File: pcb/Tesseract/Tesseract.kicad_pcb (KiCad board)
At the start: 2 copper layers, 67 x 55 mm, 31 parts, among them IC1 MAX98357AETE+T, J1 NHD-1.91-176176UBC3 Conn-1, J2 USB C Power Connector, J3 Speaker Connector, J4 RPI Power Connector, J5 LED Strip Connector, J6 RPI Signal Connector 1, J7 RPI Signal Connector 2, J8 NHD-1.91-176176UBC3 Conn-2, SW1 SW_Push, SW2 SW_Push, SW3 SW_Push, SW4 SW_Push

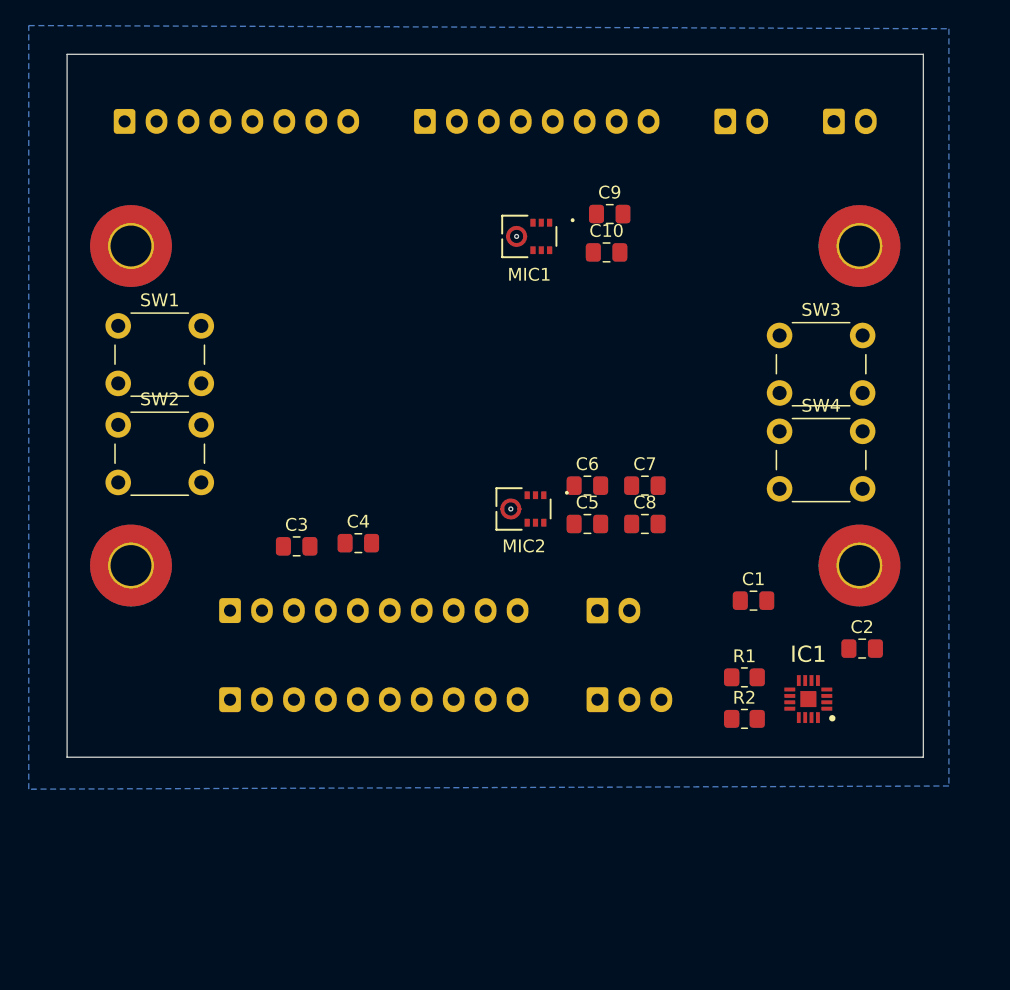
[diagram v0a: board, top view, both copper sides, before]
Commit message: Add yesterday's work to journal
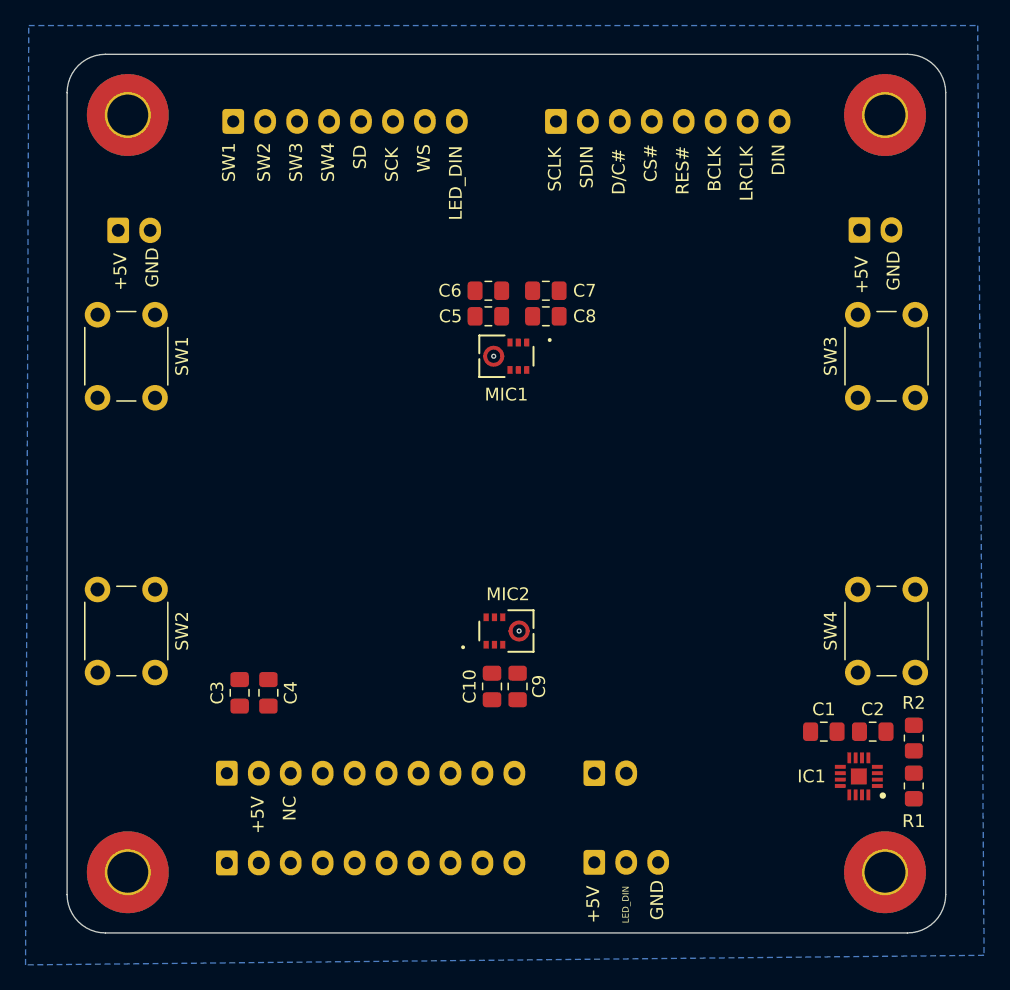
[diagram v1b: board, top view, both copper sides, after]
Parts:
- moved J4 56.6 mm to (54.0, 63.8)
- moved C9 37.7 mm to (85.2, 99.5), turned to -90 degrees
- moved C10 35.1 mm to (83.2, 99.5), turned to -90 degrees
- moved REF** 24.1 mm to (114.0, 114.0)
- moved REF** 24.0 mm to (54.8, 114.0)
- moved SW4 19.8 mm to (111.9, 98.4), turned to 90 degrees
- moved J8 19.8 mm to (62.5, 113.3)
- moved C5 18.0 mm to (83.0, 70.5)
- moved C8 18.0 mm to (87.5, 70.5)
- moved C6 17.1 mm to (83.0, 68.5)
- moved C7 17.1 mm to (87.5, 68.5)
- moved R1 15.7 mm to (116.2, 107.2), turned to -90 degrees
- moved C4 13.7 mm to (65.8, 100.0), turned to -90 degrees
- moved J2 13.5 mm to (112.0, 63.8)
- moved R2 13.3 mm to (116.2, 103.5), turned to -90 degrees
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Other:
- board size 67 x 55 mm -> 68.8 x 68.8 mm
- board text added: "+5V"
- board text added: "BCLK"
- board text added: "CS#"
- board text added: "D/C#"
- board text added: "DIN"
- board text added: "GND"
- board text added: "IC1"
- board text added: "LED_DIN"
- board text added: "LRCLK"
- board text added: "NC"
- board text added: "RES#"
- board text added: "SCK"
- board text added: "SCLK"
- board text added: "SD"
- board text added: "SDIN"
- board text added: "SW1"
- board text added: "SW2"
- board text added: "SW3"
- board text added: "SW4"
- board text added: "WS"
